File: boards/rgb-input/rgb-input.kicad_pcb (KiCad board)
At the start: 2 copper layers, 138.9 x 89.2 mm, 174 parts, among them J1 Barrel_Jack, J13 I2C, J42 INPUTS, J46 RGB, U1 ESP32-DEVKITC, U13 MCP1502, U2 MCP3208, U3 XL1509-5.0, U5 TLC5947DAP, U6 TLC5947DAP

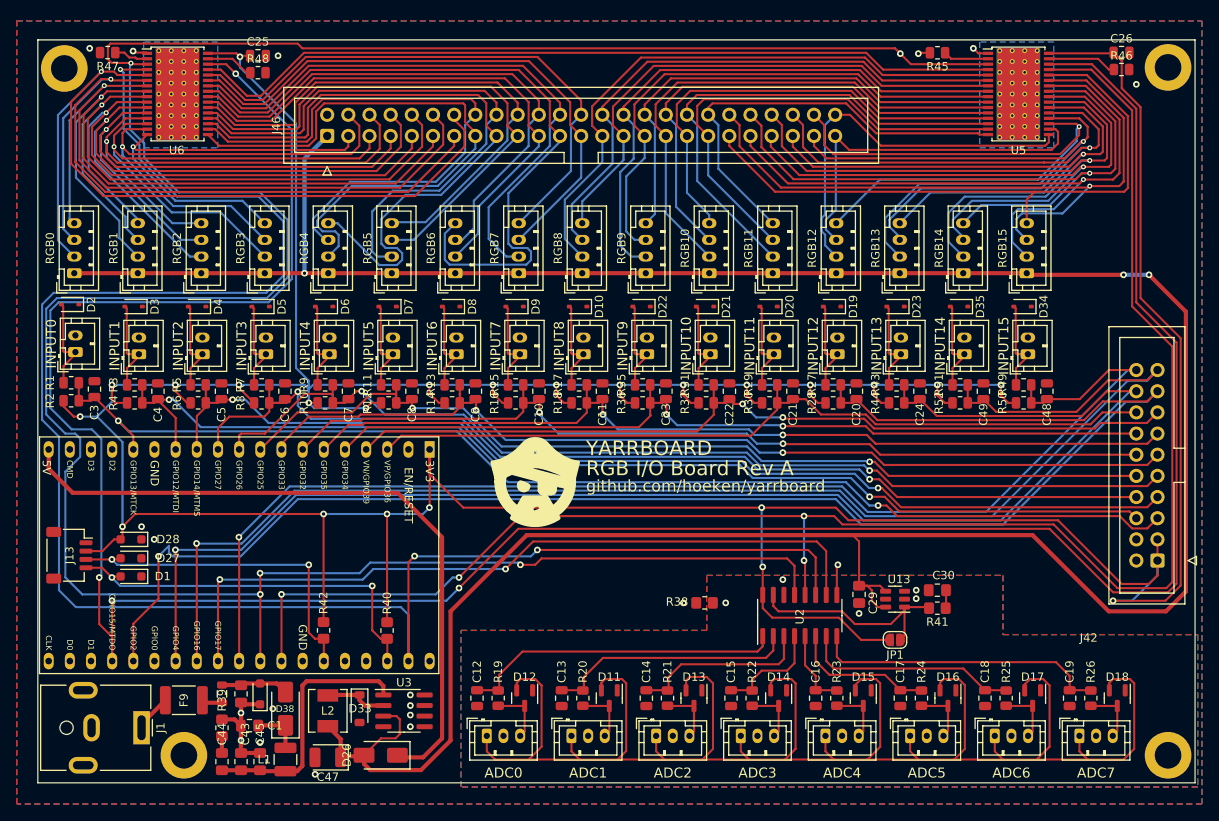
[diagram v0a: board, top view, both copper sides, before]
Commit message: various cleanups and tidying
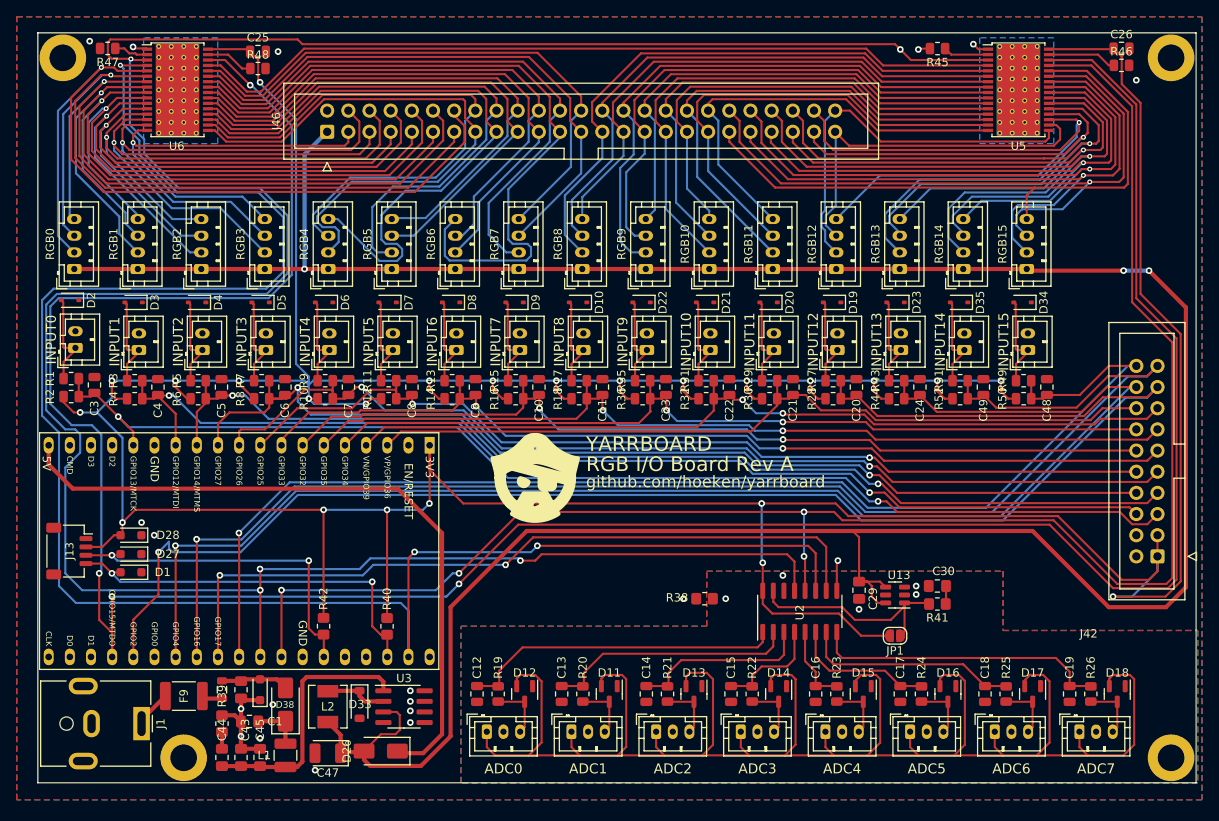
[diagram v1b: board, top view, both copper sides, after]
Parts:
- moved H3 1.29 mm to (78.0, 53.0)
- moved H4 1.20 mm to (211.0, 53.0)
- moved ADC0 0.50 mm to (128.9, 133.9)
- moved ADC1 0.50 mm to (139.0, 133.9)
- moved ADC2 0.50 mm to (149.2, 133.9)
- moved ADC3 0.50 mm to (159.4, 133.9)
- moved ADC4 0.50 mm to (169.5, 133.9)
- moved ADC5 0.50 mm to (179.7, 133.9)
- moved ADC6 0.50 mm to (189.8, 133.9)
- moved ADC7 0.50 mm to (200.0, 133.9)
- moved C1 0.50 mm to (100.4, 132.6)
- moved C10 0.50 mm to (135.1, 92.5)
- moved C11 0.50 mm to (142.8, 92.5)
- moved C12 0.50 mm to (127.7, 129.3)
- moved C13 0.50 mm to (137.9, 129.3)
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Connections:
- H1 pad 1: (no net) -> unconnected-(H1-Pad1)
- H2 pad 1: (no net) -> unconnected-(H2-Pad1)
- H3 pad 1: (no net) -> unconnected-(H3-Pad1)
- H4 pad 1: (no net) -> unconnected-(H4-Pad1)
- J1 pad MP: (no net) -> GNDD
- J13 pad MP: (no net) -> unconnected-(J13-MountPin-PadMP)
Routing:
- net /LEDS/GREEN4: track 68.4 -> 66.5 mm
- net /LEDS/BLUE4: track 79.1 -> 77.2 mm
- net /LEDS/RED4: track 70.6 -> 68.7 mm
- net /LEDS/RED5: track 69.6 -> 68.0 mm
- net /LEDS/GREEN5: track 65.9 -> 64.4 mm
- net /LEDS/BLUE5: track 65.6 -> 64.2 mm
- net /LEDS/BLUE3: track 50.1 -> 50.7 mm
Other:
- board size 138.9 x 89.2 mm -> 139 x 90 mm
